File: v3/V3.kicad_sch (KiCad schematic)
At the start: 64 parts, among them J1 Conn_01x02_Pin, J10 USB_C_Receptacle_USB2.0_16P, J11 Conn_01x02_Pin, J12 Conn_01x02_Pin, J13 Conn_01x02_Pin, J14 Conn_01x02_Pin, J2 Conn_02x07_Odd_Even, J3 Conn_01x02, J4 Conn_01x02, J5 Conn_01x02, J6 Conn_01x02, J7 Conn_01x02_Pin, J8 Conn_01x02_Pin, J9 Conn_01x02_Pin, Q1 BCX56, U1 STM32G431K6Tx, U2 MCP1802x-xx02xOT, X1 MU00525-32.768K

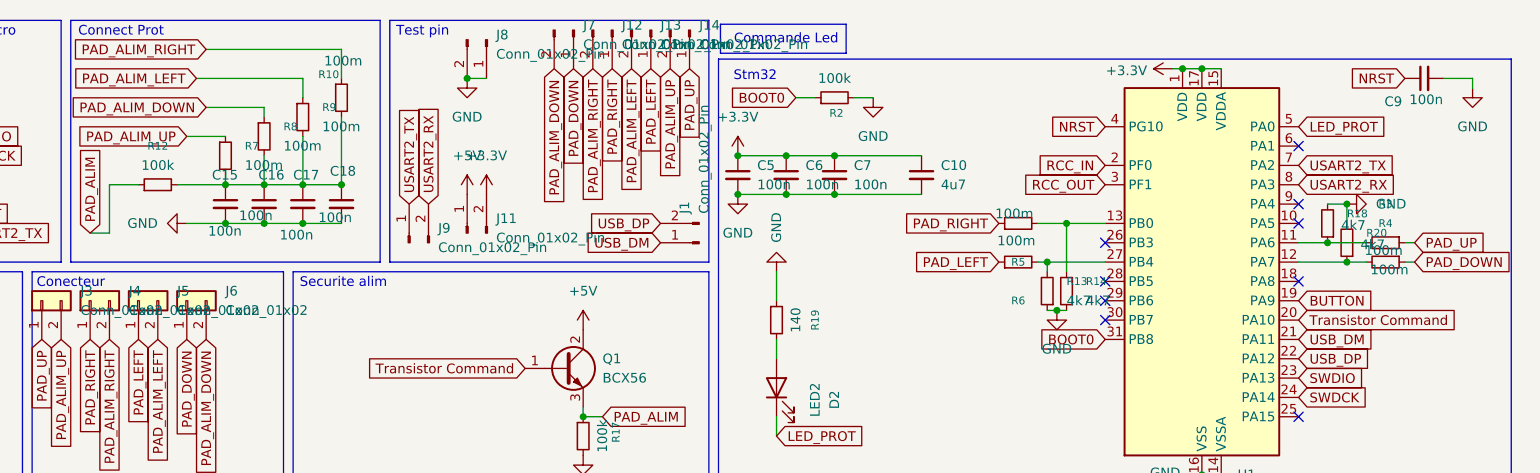
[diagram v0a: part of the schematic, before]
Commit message: Version final
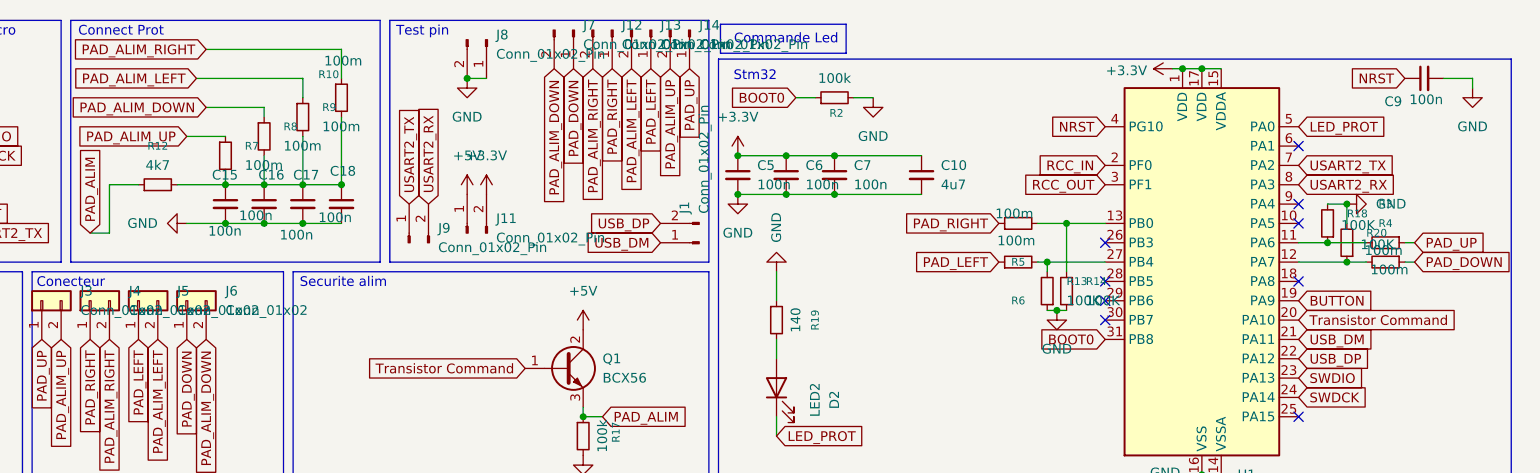
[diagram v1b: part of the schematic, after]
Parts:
- R12: value 100k -> 4k7
- R13, R14, R18, R20: value 4k7 -> 100K
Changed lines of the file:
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@@
 			)
 		)
-		(property "Value" "4k7"
+		(property "Value" "100K"
 			(at 226.06 49.5299 0)
 			(effects
@@
 			)
 		)
-		(property "Value" "4k7"
+		(property "Value" "100K"
 			(at 259.588 39.624 0)
 			(effects
@@
 			)
 		)
-		(property "Value" "100k"
+		(property "Value" "4k7"
 			(at 104.14 31.75 90)
 			(effects
@@
 			)
 		)
-		(property "Value" "4k7"
+		(property "Value" "100K"
 			(at 223.52 49.5299 0)
 			(effects
@@
 			)
 		)
-		(property "Value" "4k7"
+		(property "Value" "100K"
 			(at 262.128 42.164 0)
 			(effects

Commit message: Version final + seri
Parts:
- J10: footprint Connector_USB:USB_C_Receptacle_GCT_USB4105-xx-A_16P_TopMnt_Horizontal -> Connector_USB:USB_C_Receptacle_HRO_TYPE-C-31-M-12
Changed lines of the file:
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@@
 			)
 		)
-		(property "Footprint" "Connector_USB:USB_C_Receptacle_GCT_USB4105-xx-A_16P_TopMnt_Horizontal"
+		(property "Footprint" "Connector_USB:USB_C_Receptacle_HRO_TYPE-C-31-M-12"
 			(at 33.02 128.27 0)
 			(effects
